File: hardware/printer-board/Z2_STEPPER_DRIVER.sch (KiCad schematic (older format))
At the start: 7 parts, among them J11 MS_SELECT, J12 TO_MOTOR, U7 A4988_MODULE

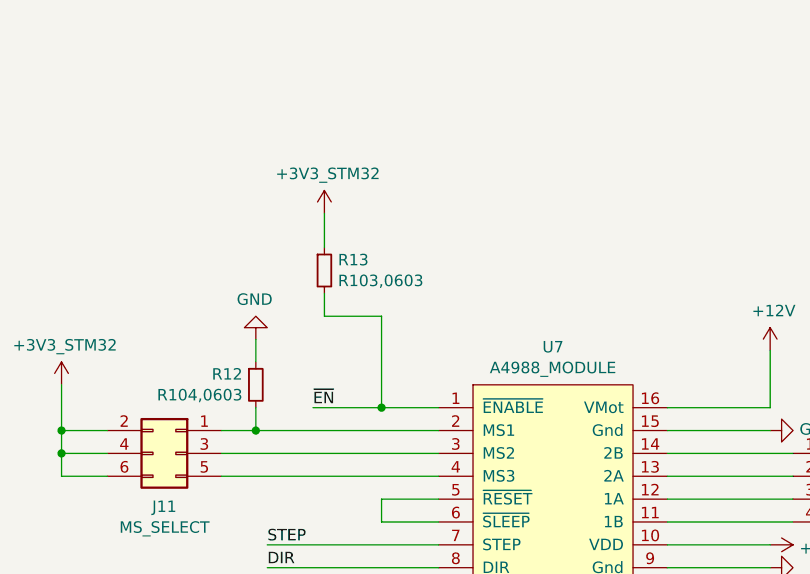
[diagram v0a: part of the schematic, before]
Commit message: update,
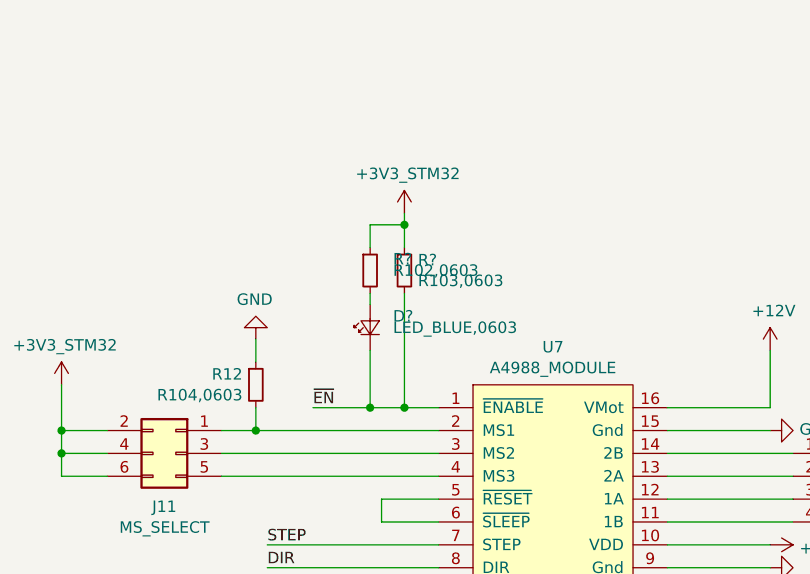
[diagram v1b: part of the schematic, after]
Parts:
- removed R13: R103,0603, Resistor_SMD:R_0603_1608Metric_Pad1.05x0.95mm_HandSolder, symbol taobao-r:R103,0603
- added D?: LED_BLUE,0603, LED_SMD:LED_0603_1608Metric_Pad1.05x0.95mm_HandSolder, symbol taobao-led:LED_BLUE,0603
- added R?: R103,0603, Resistor_SMD:R_0603_1608Metric_Pad1.05x0.95mm_HandSolder, symbol taobao-r:R103,0603
- added R?: R102,0603, Resistor_SMD:R_0603_1608Metric_Pad1.05x0.95mm_HandSolder, symbol taobao-r:R102,0603
- J12: footprint footprint-lib:s4b-ph-kl,stepper_motor_terminal -> Connector_PinHeader_2.00mm:PinHeader_1x04_P2.00mm_Vertical
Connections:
- net +3V3_STM32: now also R?.1, R?.1
- net ~EN~: now also D?.1 (K), R?.2
- new net: D?.2 (A), R?.2
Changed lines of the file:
@@
 $Descr A4 11693 8268
 encoding utf-8
-Sheet 1 34
+Sheet 8 33
 Title ""
 Date ""
@@
 F 3 "" H 5650 3200 50  0001 C CNN
 	1    5650 3150
-	1    0    0    -1
-$EndComp
-$Comp
-L taobao-r:R103,0603 R?
-U 1 1 5CC04CCC
-P 4650 2200
-AR Path="/5CC02AB8/5CC04CCC" Ref="R?"  Part="1"
-AR Path="/5CC049BB/5CC04CCC" Ref="R?"  Part="1"
-AR Path="/5CC0A4B9/5CC04CCC" Ref="R?"  Part="1"
-AR Path="/5CC0A53C/5CC04CCC" Ref="R?"  Part="1"
-AR Path="/5CC0A8C5/5CC04CCC" Ref="R?"  Part="1"
-AR Path="/5CC0A8CA/5CC04CCC" Ref="R13"  Part="1"
-AR Path="/5CC0A8CF/5CC04CCC" Ref="R?"  Part="1"
-AR Path="/5CC0AED3/5CC04CCC" Ref="R?"  Part="1"
-AR Path="/5CC04CCC" Ref="R13"  Part="1"
-F 0 "R13" H 4709 2246 50  0000 L CNN
-F 1 "R103,0603" H 4709 2155 50  0000 L CNN
-F 2 "Resistor_SMD:R_0603_1608Metric_Pad1.05x0.95mm_HandSolder" H 4650 2200 50  0001 C CNN
-F 3 "~" H 4650 2200 50  0001 C CNN
-	1    4650 2200
 	1    0    0    -1
 $EndComp
@@
 F 0 "J12" H 6980 3092 50  0000 L CNN
 F 1 "TO_MOTOR" H 6980 3001 50  0000 L CNN
-F 2 "footprint-lib:s4b-ph-kl,stepper_motor_terminal" H 6900 3100 50  0001 C CNN
+F 2 "Connector_PinHeader_2.00mm:PinHeader_1x04_P2.00mm_Vertical" H 6900 3100 50  0001 C CNN
 F 3 "~" H 6900 3100 50  0001 C CNN
 	1    6900 3100
@@
 Text Label 4600 2800 0    50   ~ 0
 ~EN~
-Wire Wire Line
-	4600 2800 4900 2800
-Wire Wire Line
-	4650 1950 4650 2100
-Wire Wire Line
-	4650 2300 4650 2400
-Wire Wire Line
-	4650 2400 4900 2400
-Wire Wire Line
-	4900 2400 4900 2800
-Connection ~ 4900 2800
-Wire Wire Line
-	4900 2800 5150 2800
 Wire Wire Line
 	3500 2900 3700 2900
@@
 $Comp
 L taobao-components:+3V3_STM32 #PWR?
-U 1 1 5CC40AF8
-P 4650 1950
-F 0 "#PWR?" H 4650 1800 50  0001 C CNN
-F 1 "+3V3_STM32" H 4665 2123 50  0000 C CNN
-F 2 "" H 4650 1950 50  0001 C CNN
-F 3 "" H 4650 1950 50  0001 C CNN
-	1    4650 1950
-	1    0    0    -1
-$EndComp
-$Comp
-L taobao-components:+3V3_STM32 #PWR?
 U 1 1 5CC40B53
 P 3500 2700
@@
 	0    1    1    0
 $EndComp
+Wire Wire Line
+	4600 2800 4850 2800
+$Comp
+L taobao-r:R103,0603 R?
+U 1 1 5CC5B1C2
+P 5000 2200
+AR Path="/5CC02AB8/5CC5B1C2" Ref="R?"  Part="1"
+AR Path="/5CC049BB/5CC5B1C2" Ref="R?"  Part="1"
+AR Path="/5CC0A4B9/5CC5B1C2" Ref="R?"  Part="1"
+AR Path="/5CC0A53C/5CC5B1C2" Ref="R?"  Part="1"
+AR Path="/5CC0A8C5/5CC5B1C2" Ref="R?"  Part="1"
+AR Path="/5CC0A8CA/5CC5B1C2" Ref="R?"  Part="1"
+AR Path="/5CC0A8CF/5CC5B1C2" Ref="R?"  Part="1"
+AR Path="/5CC0AEC9/5CC5B1C2" Ref="R?"  Part="1"
+F 0 "R?" H 5059 2246 50  0000 L CNN
+F 1 "R103,0603" H 5059 2155 50  0000 L CNN
+F 2 "Resistor_SMD:R_0603_1608Metric_Pad1.05x0.95mm_HandSolder" H 5000 2200 50  0001 C CNN
+F 3 "~" H 5000 2200 50  0001 C CNN
+	1    5000 2200
+	1    0    0    -1
+$EndComp
+Wire Wire Line
+	5000 1950 5000 2000
+$Comp
+L taobao-components:+3V3_STM32 #PWR?
+U 1 1 5CC5B1CA
+P 5000 1950
+F 0 "#PWR?" H 5000 1800 50  0001 C CNN
+F 1 "+3V3_STM32" H 5015 2123 50  0000 C CNN
+F 2 "" H 5000 1950 50  0001 C CNN
+F 3 "" H 5000 1950 50  0001 C CNN
+	1    5000 1950
+	1    0    0    -1
+$EndComp
+$Comp
+L taobao-r:R102,0603 R?
+U 1 1 5CC5B1D0
+P 4850 2200
+AR Path="/5CC15C35/5CC5B1D0" Ref="R?"  Part="1"
+AR Path="/5CC0AEC9/5CC5B1D0" Ref="R?"  Part="1"
+F 0 "R?" H 4950 2250 50  0000 L CNN
+F 1 "R102,0603" H 4950 2200 50  0000 L CNN
+F 2 "Resistor_SMD:R_0603_1608Metric_Pad1.05x0.95mm_HandSolder" H 4850 2200 50  0001 C CNN
+F 3 "~" H 4850 2200 50  0001 C CNN
+	1    4850 2200
+	1    0    0    -1
+$EndComp
+$Comp
+L taobao-led:LED_BLUE,0603 D?
+U 1 1 5CC5B1D7
+P 4850 2450
+AR Path="/5CC15C35/5CC5B1D7" Ref="D?"  Part="1"
+AR Path="/5CC0AEC9/5CC5B1D7" Ref="D?"  Part="1"
+F 0 "D?" V 4900 2350 50  0000 R CNN
+F 1 "LED_BLUE,0603" V 4850 2350 50  0000 R CNN
+F 2 "LED_SMD:LED_0603_1608Metric_Pad1.05x0.95mm_HandSolder" V 4850 2450 50  0001 C CNN
+F 3 "" V 4850 2450 50  0001 C CNN
+	1    4850 2450
+	0    -1   -1   0
+$EndComp
+Wire Wire Line
+	4850 2300 4850 2350
+Wire Wire Line
+	4850 2100 4850 2000
+Wire Wire Line
+	5000 2300 5000 2800
+Wire Wire Line
+	4850 2550 4850 2800
+Connection ~ 5000 2000
+Wire Wire Line
+	5000 2000 5000 2100
+Wire Wire Line
+	4850 2000 5000 2000
+Connection ~ 4850 2800
+Wire Wire Line
+	4850 2800 5000 2800
+Connection ~ 5000 2800
+Wire Wire Line
+	5000 2800 5150 2800
 $EndSCHEMATC
